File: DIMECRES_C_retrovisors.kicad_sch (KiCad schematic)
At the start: 1 part, among them U1 PIC18F258-xSO

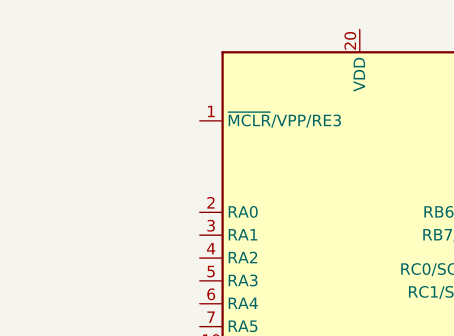
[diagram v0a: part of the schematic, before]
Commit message: prueba 2
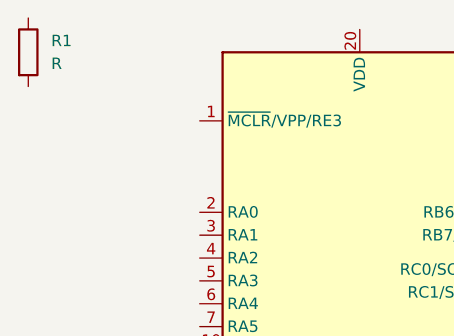
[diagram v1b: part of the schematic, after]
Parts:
- added R1: R, symbol Device:R
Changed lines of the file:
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@@
+		)
+	)
+	(symbol
+		(lib_id "Device:R")
+		(at 110.49 60.96 0)
+		(unit 1)
+		(exclude_from_sim no)
+		(in_bom yes)
+		(on_board yes)
+		(dnp no)
+		(fields_autoplaced yes)
+		(property "Reference" "R1"
+			(at 113.03 59.6899 0)
+			(effects
+				(font
+					(size 1.27 1.27)
+				)
+				(justify left)
+			)
+		)
+		(property "Value" "R"
+			(at 113.03 62.2299 0)
+			(effects
+				(font
+					(size 1.27 1.27)
+				)
+				(justify left)
+			)
+		)
+		(property "Footprint" ""
+			(at 108.712 60.96 90)
+			(effects
+				(font
+					(size 1.27 1.27)
+				)
+				(hide yes)
+			)
+		)
+		(property "Datasheet" "~"
+			(at 110.49 60.96 0)
+			(effects
+				(font
+					(size 1.27 1.27)
+				)
+				(hide yes)
+			)
+		)
+		(property "Description" "Resistor"
+			(at 110.49 60.96 0)
+			(effects
+				(font
+					(size 1.27 1.27)
+				)
+				(hide yes)
+			)
+		)
+		(pin "1"
+		)
+		(pin "2"
+		)
+		(instances
+			(project ""
+				(path "/c3f67613-7195-4d14-ab28-355c40c698ae"
+					(reference "R1")
+					(unit 1)
+				)
+			)
 		)
 	)

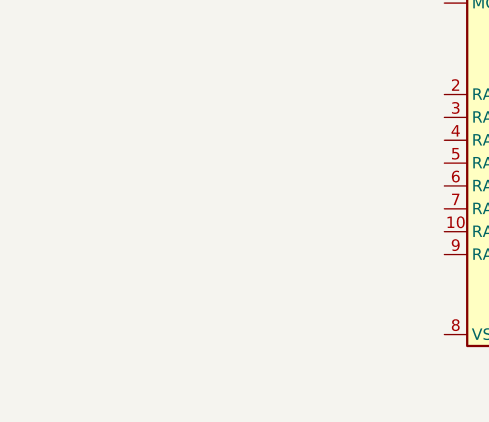
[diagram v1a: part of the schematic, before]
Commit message: ¿?
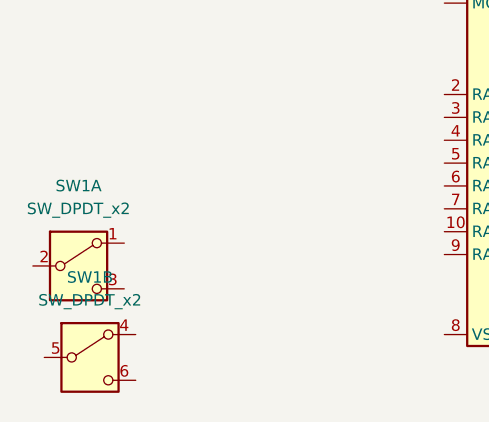
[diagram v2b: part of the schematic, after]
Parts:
- added SW1: SW_DPDT_x2, symbol Switch:SW_DPDT_x2
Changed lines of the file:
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@@
+	)
+	(symbol
+		(lib_id "Switch:SW_DPDT_x2")
+		(at 88.9 97.79 0)
+		(unit 1)
+		(exclude_from_sim no)
+		(in_bom yes)
+		(on_board yes)
+		(dnp no)
+		(fields_autoplaced yes)
+		(property "Reference" "SW1"
+			(at 88.9 88.9 0)
+			(effects
+				(font
+					(size 1.27 1.27)
+				)
+			)
+		)
+		(property "Value" "SW_DPDT_x2"
+			(at 88.9 91.44 0)
+			(effects
+				(font
+					(size 1.27 1.27)
+				)
+			)
+		)
+		(property "Footprint" ""
+			(at 88.9 97.79 0)
+			(effects
+				(font
+					(size 1.27 1.27)
+				)
+				(hide yes)
+			)
+		)
+		(property "Datasheet" "~"
+			(at 88.9 97.79 0)
+			(effects
+				(font
+					(size 1.27 1.27)
+				)
+				(hide yes)
+			)
+		)
+		(property "Description" "Switch, dual pole double throw, separate symbols"
+			(at 88.9 97.79 0)
+			(effects
+				(font
+					(size 1.27 1.27)
+				)
+				(hide yes)
+			)
+		)
+		(pin "5"
+		)
+		(pin "2"
+		)
+		(pin "1"
+		)
+		(pin "6"
+		)
+		(pin "3"
+		)
+		(pin "4"
+		)
+		(instances
+			(project ""
+				(path "/c3f67613-7195-4d14-ab28-355c40c698ae"
+					(reference "SW1")
+					(unit 1)
+				)
+			)
+		)
+	)
+	(symbol
+		(lib_id "Switch:SW_DPDT_x2")
+		(at 90.17 107.95 0)
+		(unit 2)
+		(exclude_from_sim no)
+		(in_bom yes)
+		(on_board yes)
+		(dnp no)
+		(fields_autoplaced yes)
+		(property "Reference" "SW1"
+			(at 90.17 99.06 0)
+			(effects
+				(font
+					(size 1.27 1.27)
+				)
+			)
+		)
+		(property "Value" "SW_DPDT_x2"
+			(at 90.17 101.6 0)
+			(effects
+				(font
+					(size 1.27 1.27)
+				)
+			)
+		)
+		(property "Footprint" ""
+			(at 90.17 107.95 0)
+			(effects
+				(font
+					(size 1.27 1.27)
+				)
+				(hide yes)
+			)
+		)
+		(property "Datasheet" "~"
+			(at 90.17 107.95 0)
+			(effects
+				(font
+					(size 1.27 1.27)
+				)
+				(hide yes)
+			)
+		)
+		(property "Description" "Switch, dual pole double throw, separate symbols"
+			(at 90.17 107.95 0)
+			(effects
+				(font
+					(size 1.27 1.27)
+				)
+				(hide yes)
+			)
+		)
+		(pin "5"
+		)
+		(pin "2"
+		)
+		(pin "1"
+		)
+		(pin "6"
+		)
+		(pin "3"
+		)
+		(pin "4"
+		)
+		(instances
+			(project ""
+				(path "/c3f67613-7195-4d14-ab28-355c40c698ae"
+					(reference "SW1")
+					(unit 2)
+				)
+			)
+		)
 	)
 	(symbol

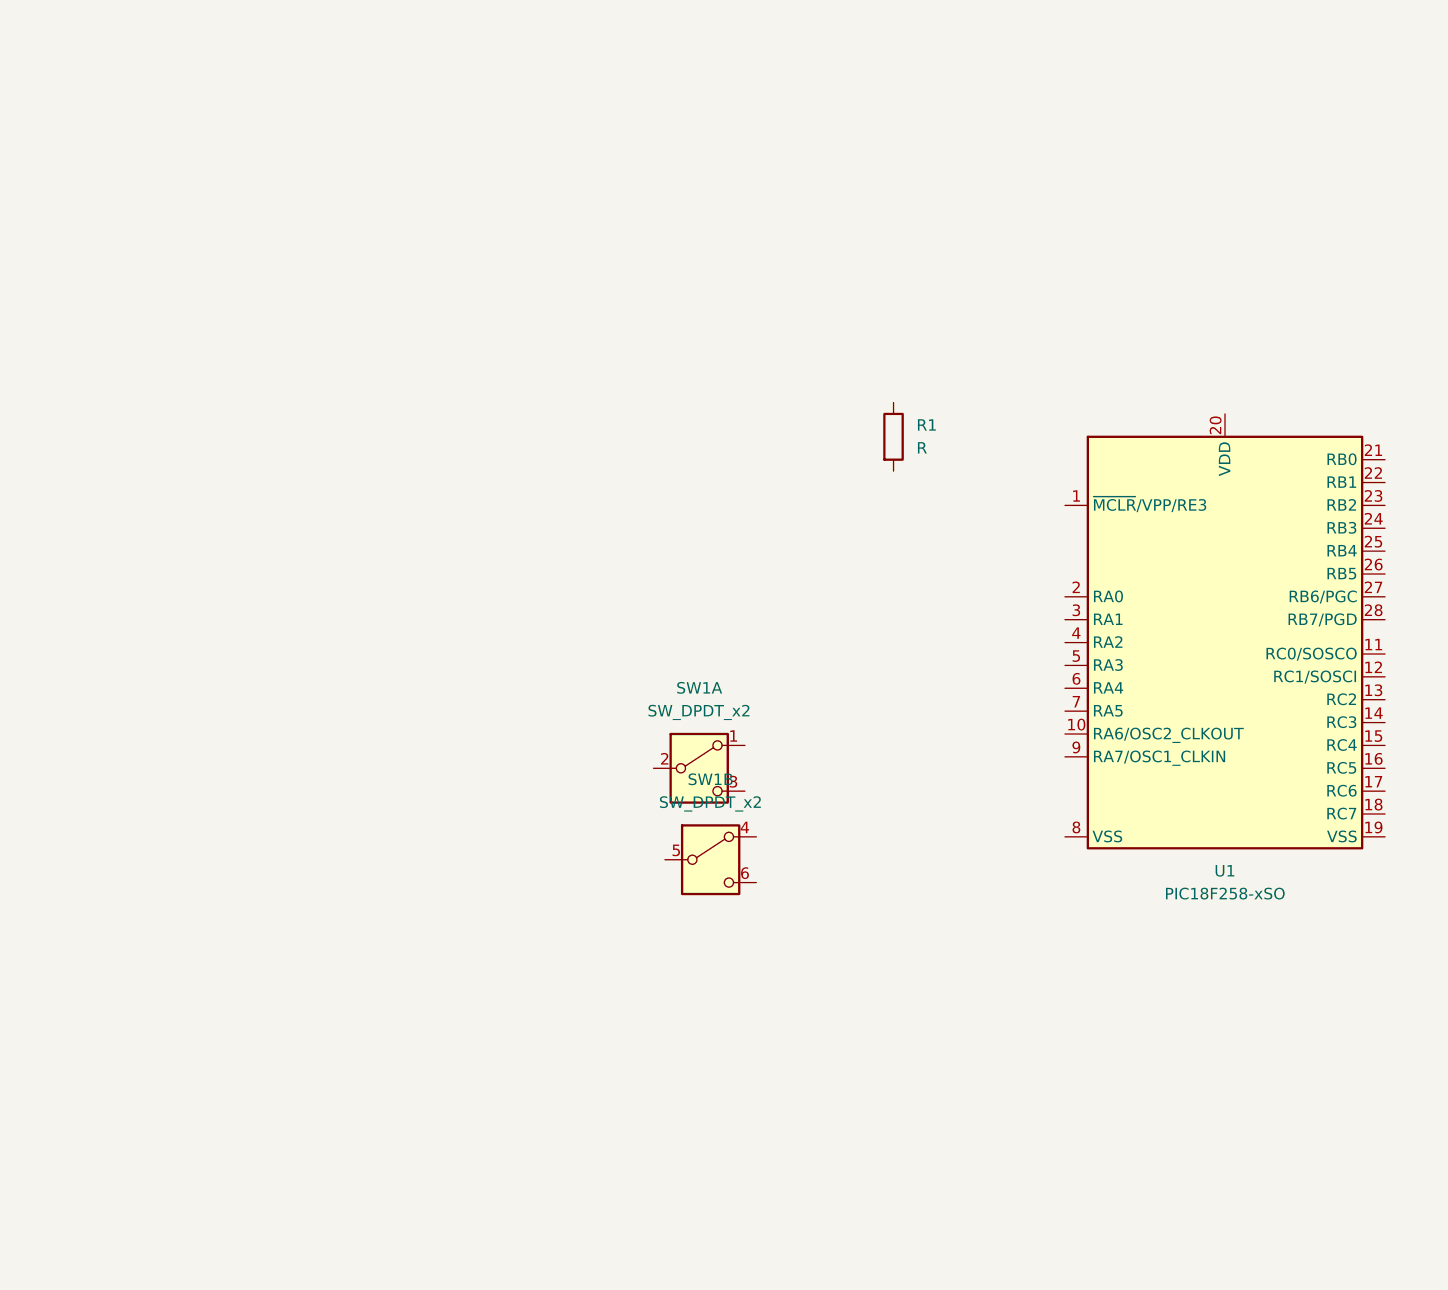
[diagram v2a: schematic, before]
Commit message: 1/2Etapa reguladora
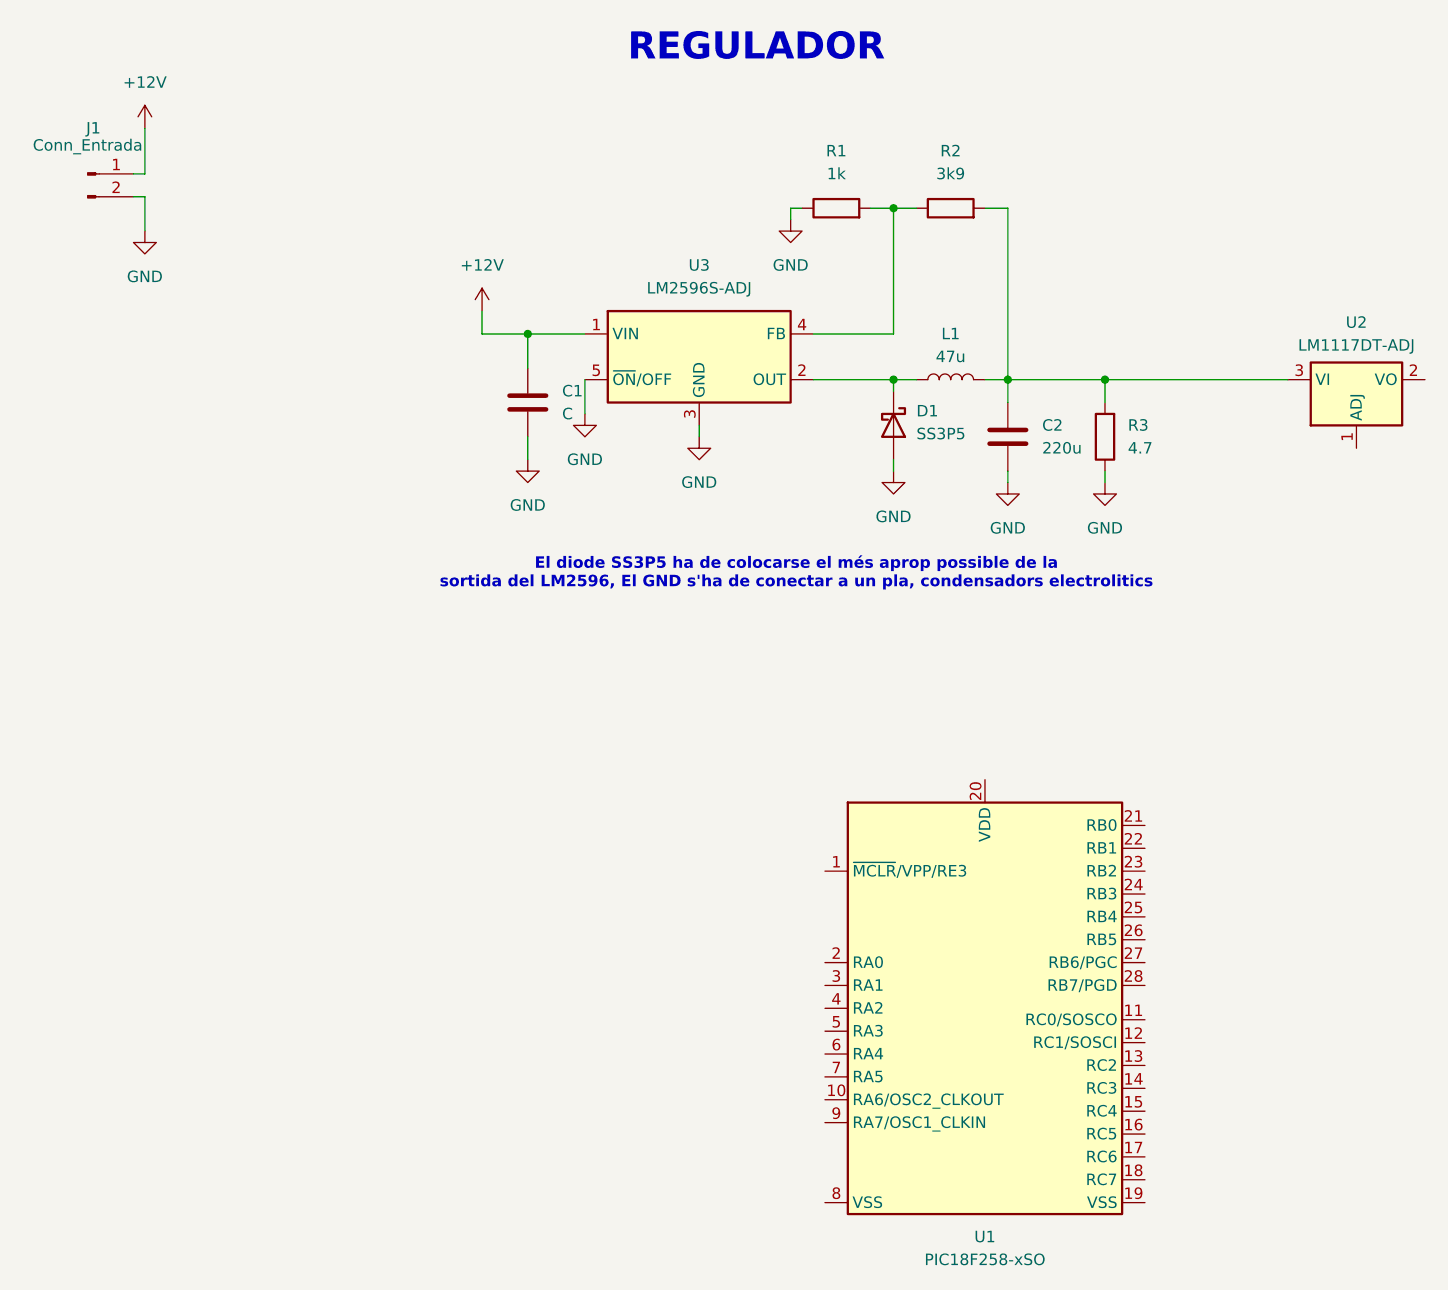
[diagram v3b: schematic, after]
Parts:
- removed SW1: SW_DPDT_x2, symbol Switch:SW_DPDT_x2
- added C1: C, symbol Device:C
- added C2: 220u, symbol Device:C
- added D1: SS3P5, symbol PracticasKiCad:SS3P5
- added J1: Conn_Entrada, symbol Connector:Conn_01x02_Pin
- added L1: 47u, symbol Device:L
- added R2: 3k9, symbol Device:R
- added R3: 4.7, symbol Device:R
- added U2: LM1117DT-ADJ, Package_TO_SOT_SMD:TO-252-3_TabPin2, symbol Regulator_Linear:LM1117DT-ADJ
- added U3: LM2596S-ADJ, Package_TO_SOT_SMD:TO-263-5_TabPin3, symbol Regulator_Switching:LM2596S-ADJ
- R1: value R -> 1k
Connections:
- net GND: now reaches R1.1
- net GND: now also C1.2, C2.2, D1.2 (A), J1.2 (Pin_2), R3.1, U3.3 (GND), U3.5 (~{ON}/OFF)
- net at R1.2: now also R2.1, U3.4 (FB)
- new net: C2.1, L1.2, R2.2, R3.2, U2.3 (VI)
- new net: D1.1 (K), L1.1, U3.2 (OUT)
- new net +12V: C1.1, J1.1 (Pin_1), U3.1 (VIN)
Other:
- note added: "El diode SS3P5 ha de colocarse el més aprop possible de la sortida del LM2596, El GND s'ha de conectar a un pla, condensadors electrolitics"
- note added: "REGULADOR"
- moved on the sheet: R1, U1

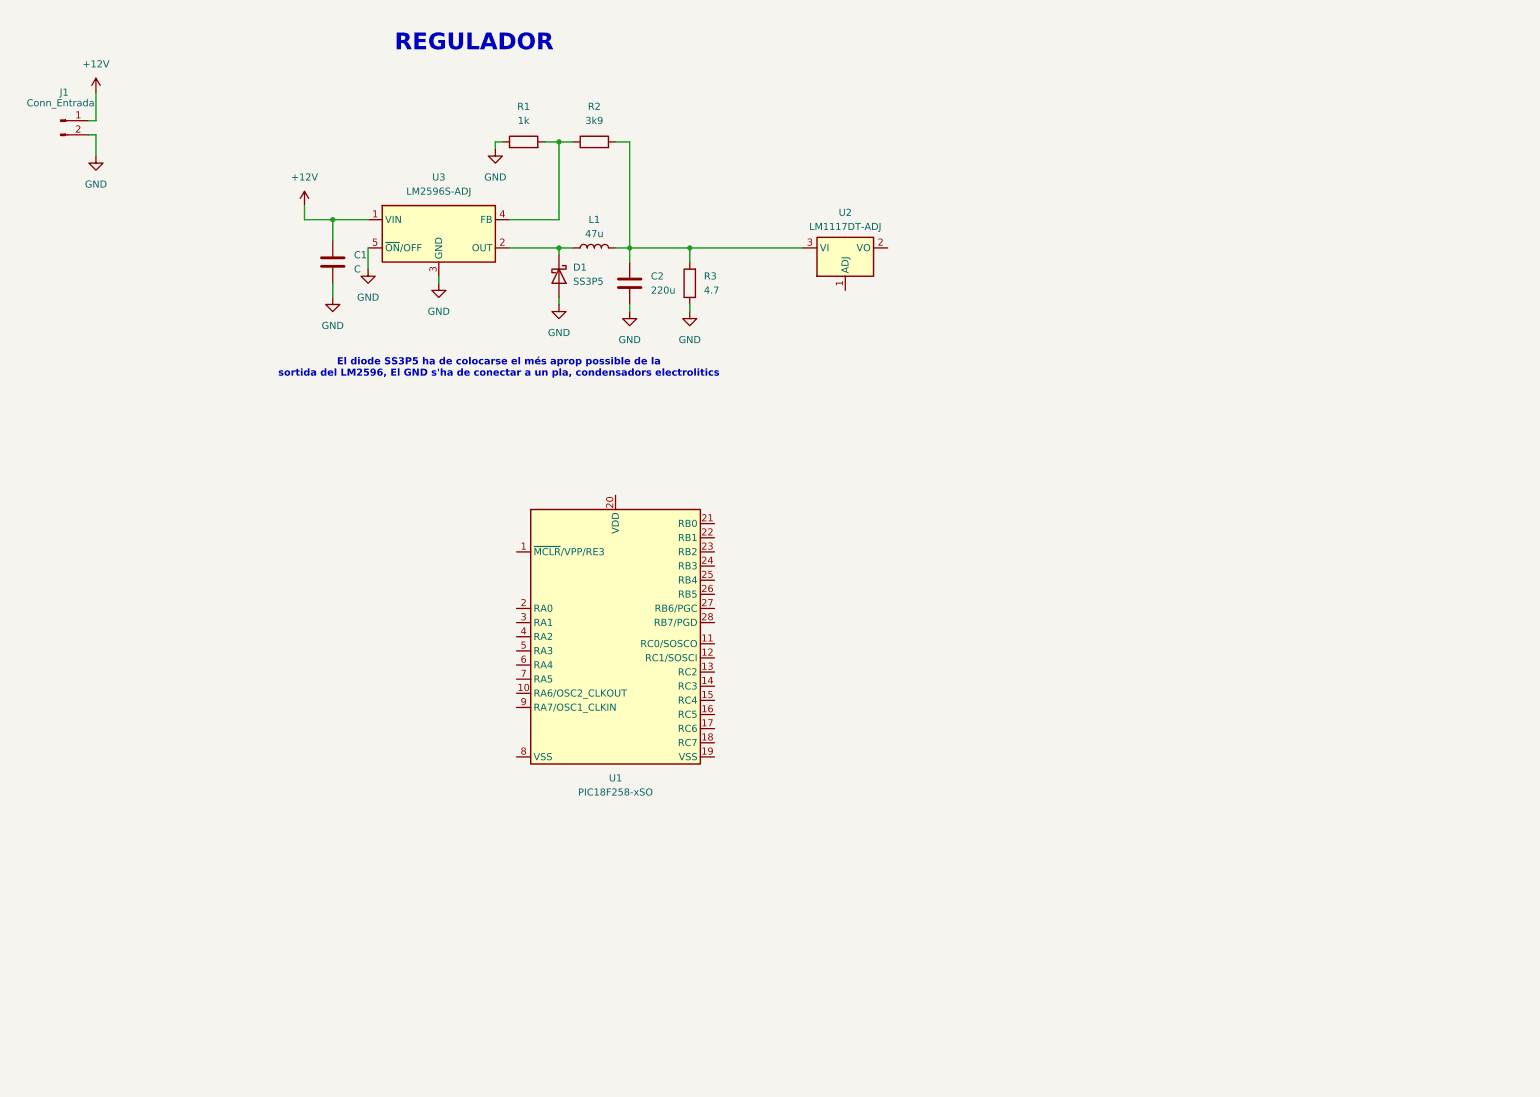
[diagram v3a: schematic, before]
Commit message: Regulador+1/3 Driver
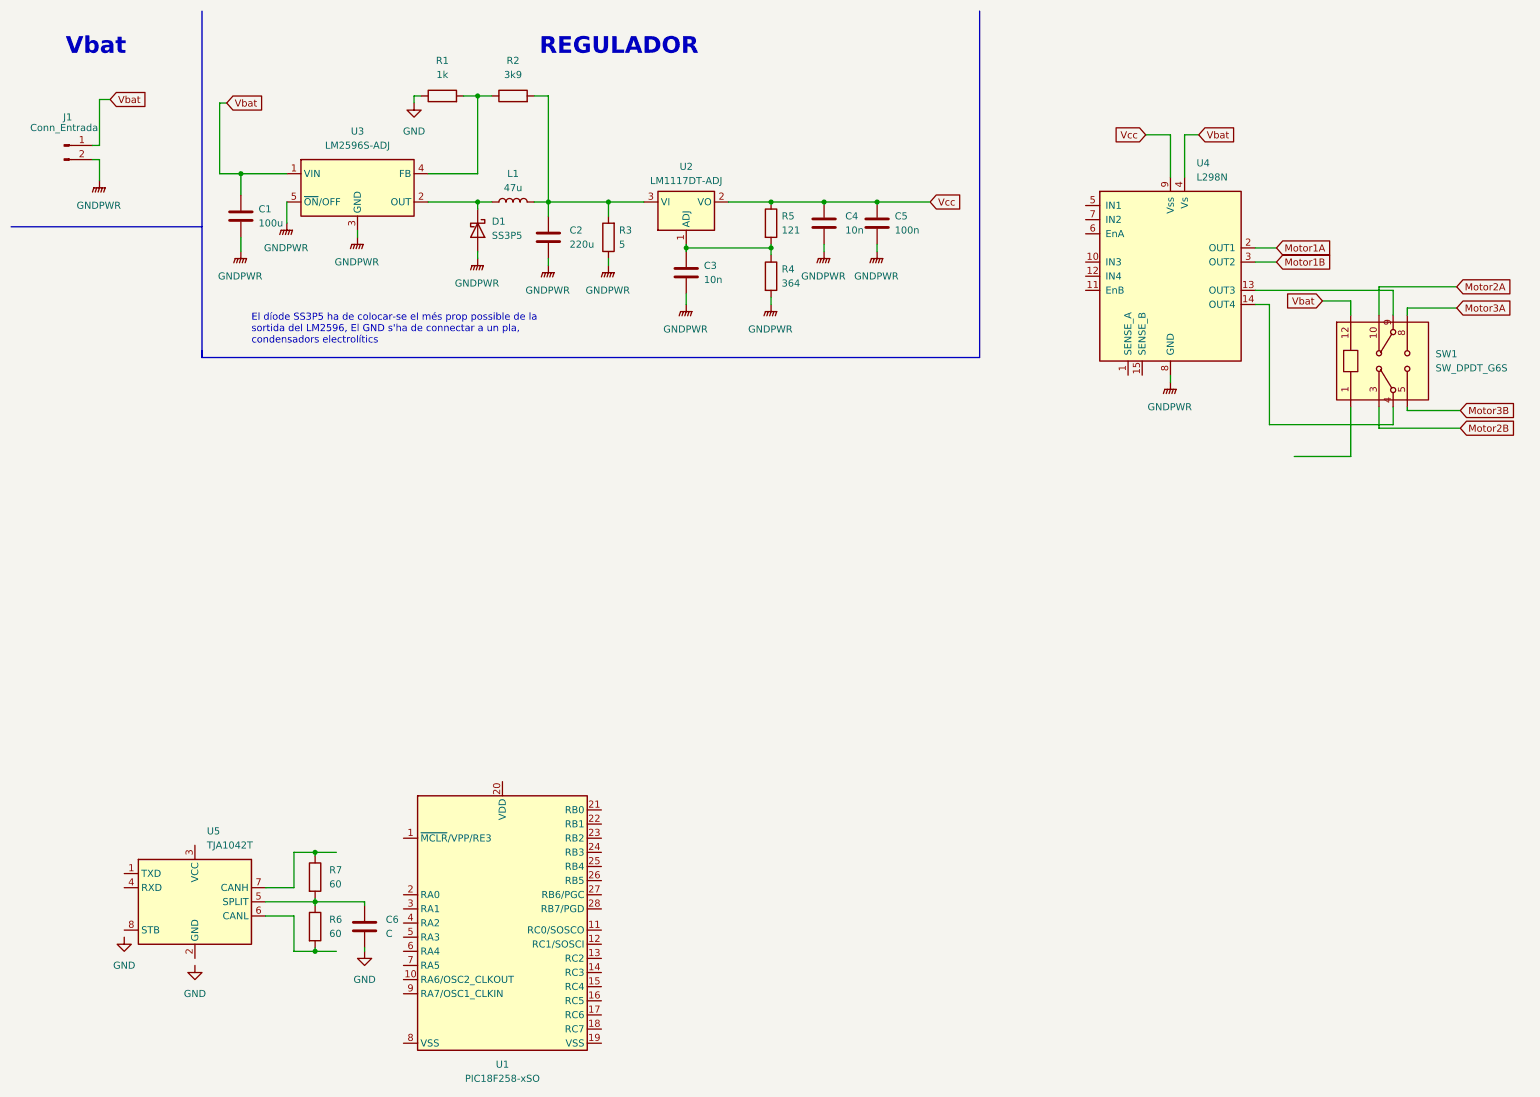
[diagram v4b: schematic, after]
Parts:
- added C3, C4: 10n, symbol Device:C
- added C5: 100n, symbol Device:C
- added C6: C, symbol Device:C
- added R4: 364, symbol Device:R
- added R5: 121, symbol Device:R
- added R6, R7: 60, symbol Device:R
- added SW1: SW_DPDT_G6S, symbol PracticasKiCad:SW_DPDT_G6S
- added U4: L298N, Package_TO_SOT_THT:TO-220-15_P2.54x2.54mm_StaggerOdd_Lead4.58mm_Vertical, symbol Driver_Motor:L298N
- added U5: TJA1042T, Package_SO:SOIC-8_3.9x4.9mm_P1.27mm, symbol Interface_CAN_LIN:TJA1042T
- C1: value C -> 100u
- R3: value 4.7 -> 5
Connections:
- net GND: now also C6.2; no longer C1.2, C2.2, D1.2 (A), J1.2 (Pin_2), R3.1, U3.3 (GND), U3.5 (~{ON}/OFF)
- net at U2.1 (ADJ): now also C3.1, R4.1, R5.2
- net Vcc: now reaches U2.2 (VO)
- net Vcc: now also C4.1, C5.1, R5.1, U4.9 (Vss)
- net +12V renamed Vbat
- net Vbat: now also SW1.12 (Cnt2), U4.4 (Vs)
- new net: C6.1, R6.1, R7.2, U5.5 (SPLIT)
- new net: R6.2, U5.6 (CANL)
- new net: R7.1, U5.7 (CANH)
- new net: SW1.9 (In2), U4.13 (OUT3)
- new net: SW1.4 (In1), U4.14 (OUT4)
- new net GNDPWR: C1.2, C2.2, C3.2, C4.2, C5.2, D1.2 (A), J1.2 (Pin_2), R3.1, R4.2, U3.3 (GND), U3.5 (~{ON}/OFF), U4.8 (GND)
- new net Motor1A: U4.2 (OUT1)
- new net Motor1B: U4.3 (OUT2)
- new net Motor2A: SW1.10 (Out2A)
- new net Motor2B: SW1.3 (Out1A)
- new net Motor3A: SW1.8 (Out2B)
- new net Motor3B: SW1.5 (Out1B)
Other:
- note added: "El díode SS3P5 ha de colocar-se el més prop possible de la sortida del LM2596, El GND s'ha de connectar a un pla, condensadors electrolítics"
- note added: "Vbat"
- note removed: "El diode SS3P5 ha de colocarse el més aprop possible de la sortida del LM2596, El GND s'ha de conectar a un pla, condensadors electrolitics"
- moved on the sheet: C1, C2, D1, J1, L1, R1, R2, R3, U1, U2, U3
